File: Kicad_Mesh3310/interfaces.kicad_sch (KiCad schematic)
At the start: 52 parts, among them J5 Vibrator, J6 Buzzer, J7 Display, Q4 BSS138, Q5 BSS138, Q6 IRLML6401, Q7 BSS138

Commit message: RF designing
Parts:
- C16, C17: footprint Capacitor_Tantalum_SMD:CP_EIA-3528-21_Kemet-B -> Capacitor_Tantalum_SMD:CP_EIA-1608-08_AVX-J
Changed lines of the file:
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@@
 			)
 		)
-		(property "Footprint" "Capacitor_Tantalum_SMD:CP_EIA-3528-21_Kemet-B"
+		(property "Footprint" "Capacitor_Tantalum_SMD:CP_EIA-1608-08_AVX-J"
 			(at 229.5652 135.89 0)
 			(effects
@@
 			)
 		)
-		(property "Footprint" "Capacitor_Tantalum_SMD:CP_EIA-3528-21_Kemet-B"
+		(property "Footprint" "Capacitor_Tantalum_SMD:CP_EIA-1608-08_AVX-J"
 			(at 248.6152 125.73 0)
 			(effects

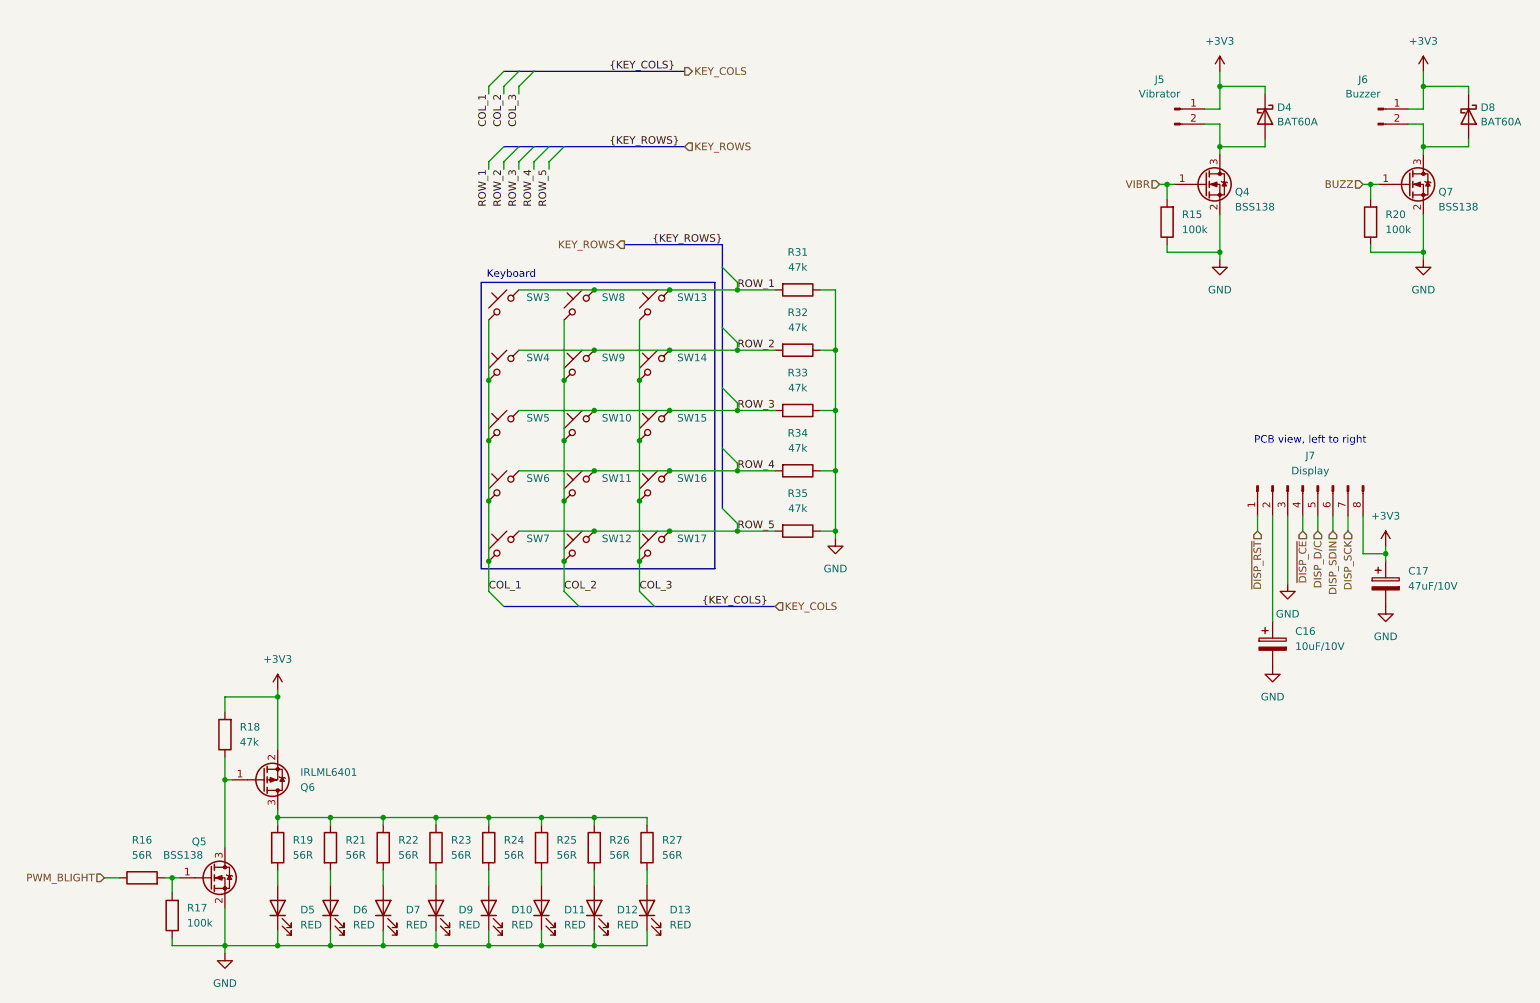
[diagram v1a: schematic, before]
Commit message: cleanup
schematic cleanup
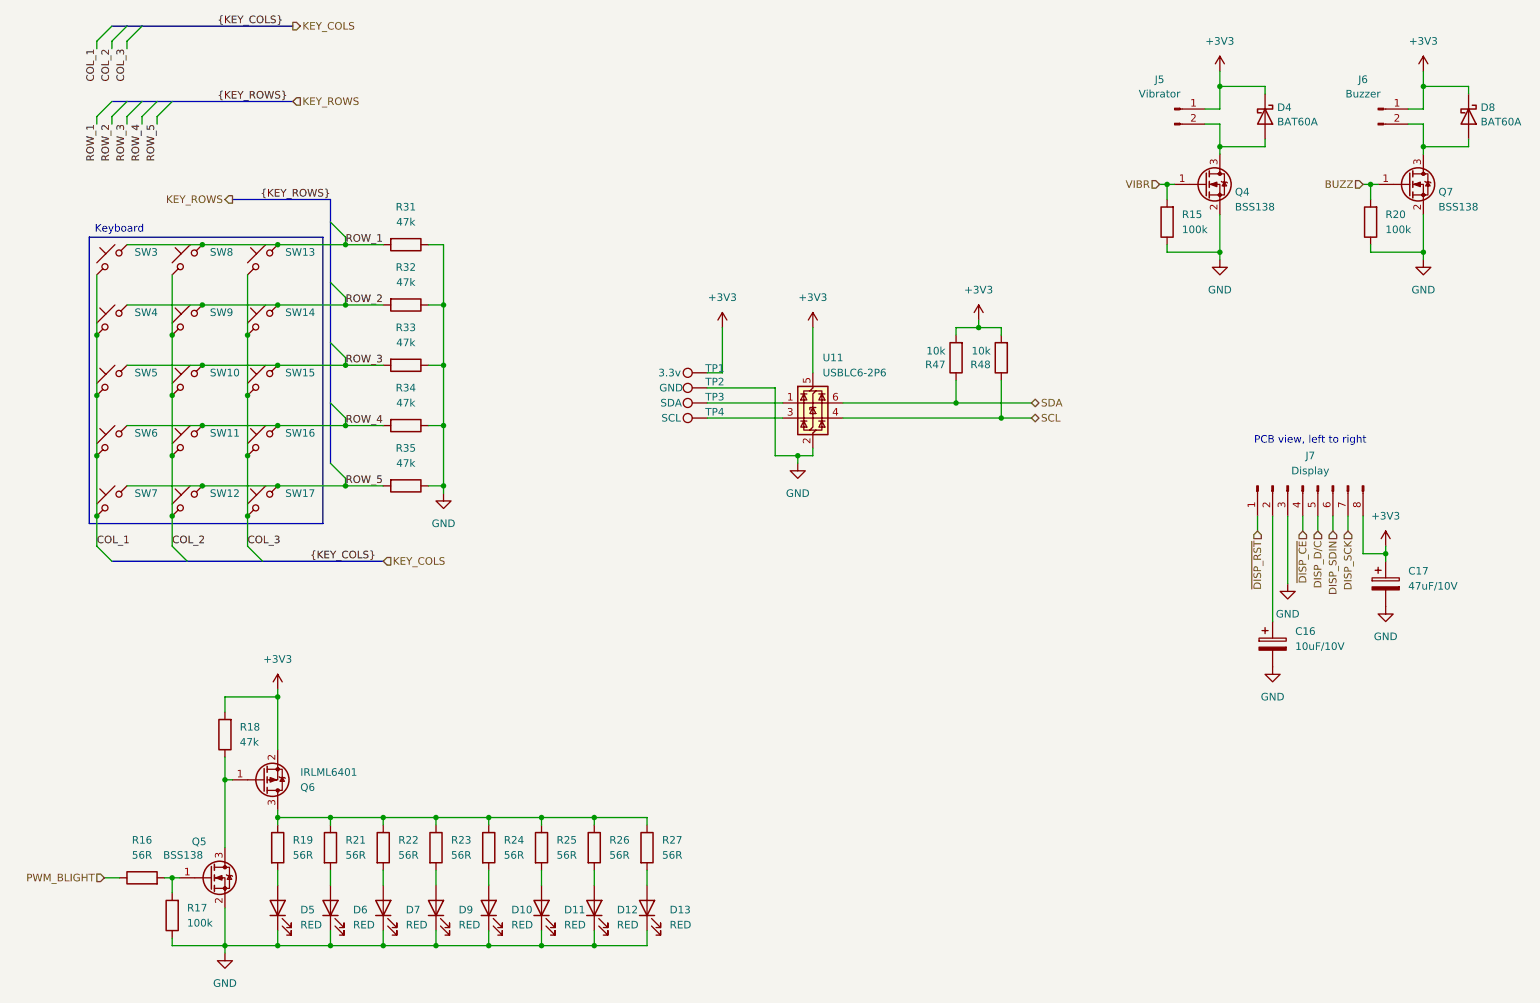
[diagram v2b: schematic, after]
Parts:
- added R47, R48: 10k, Resistor_SMD:R_0402_1005Metric, symbol symbols:R
- added TP1: 3.3v, TestPoint:TestPoint_Pad_D1.5mm, symbol Connector:TestPoint
- added TP2: GND, TestPoint:TestPoint_Pad_D1.5mm, symbol Connector:TestPoint
- added TP3: SDA, TestPoint:TestPoint_Pad_D1.5mm, symbol Connector:TestPoint
- added TP4: SCL, TestPoint:TestPoint_Pad_D1.5mm, symbol Connector:TestPoint
- added U11: USBLC6-2P6, Package_TO_SOT_SMD:SOT-666, symbol Power_Protection:USBLC6-2P6
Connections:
- net +3V3: now also R47.2, R48.2, TP1.1, U11.5 (VBUS)
- net GND: now also TP2.1, U11.2 (GND)
- new net: TP4.1, U11.3 (I/O2)
- new net: TP3.1, U11.1 (I/O1)
- new net SCL: R48.1, U11.4 (I/O2)
- new net SDA: R47.1, U11.6 (I/O1)
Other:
- moved on the sheet: R31, R32, R33, R34, R35, SW10, SW11, SW12, SW13, SW14, SW15, SW16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
